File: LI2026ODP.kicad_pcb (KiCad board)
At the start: 4 copper layers, 19.8 x 40.1 mm, 33 parts, among them J1 9-1437539-2, J2 Conn_01x05_Male, U1 LM2936MPX-3.0_NOPB, U2 STM32G0B1KET6, U3 max6921aui

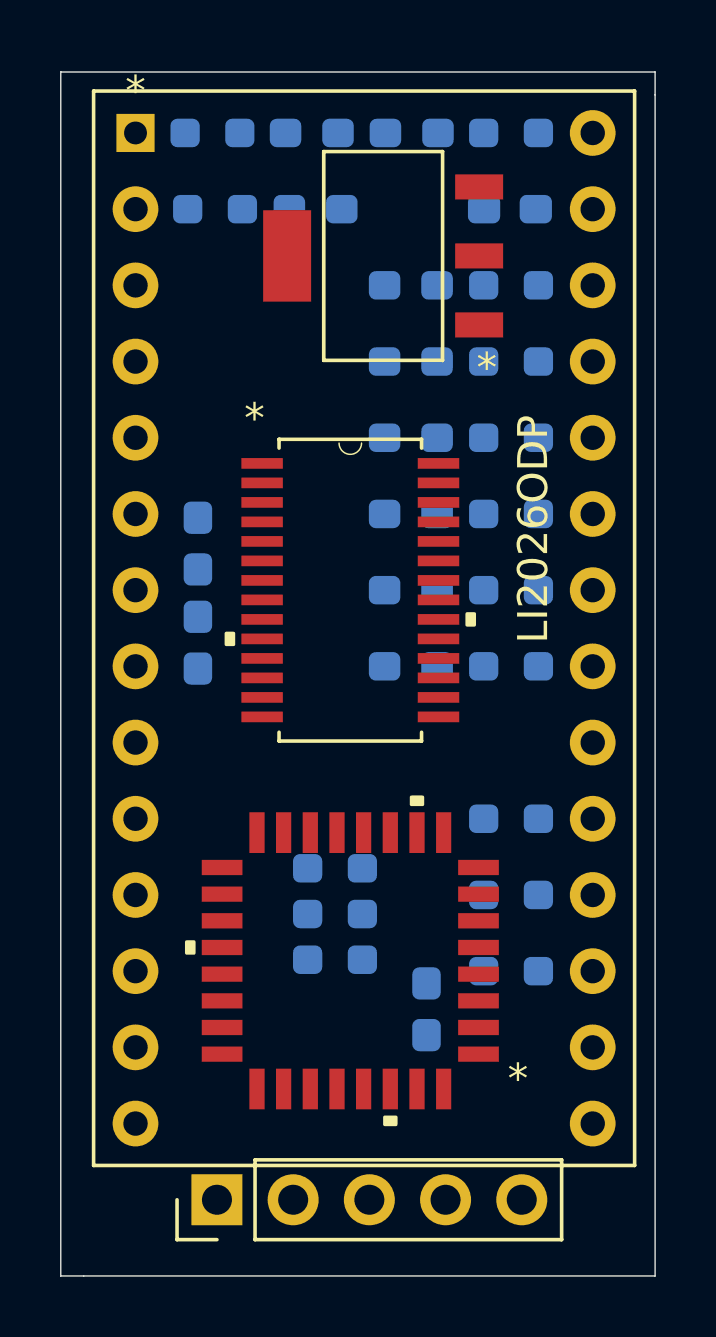
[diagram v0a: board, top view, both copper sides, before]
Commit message: layout finished.
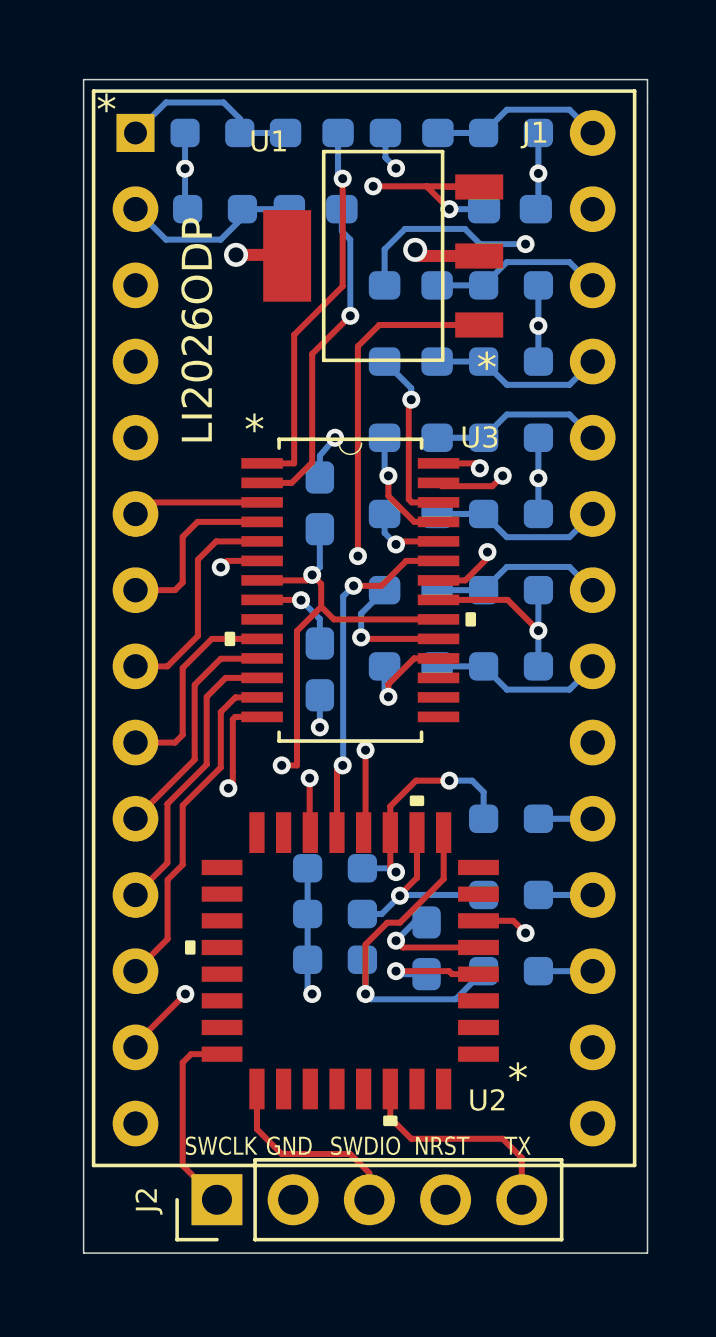
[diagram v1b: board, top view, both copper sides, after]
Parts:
- moved C3 4.28 mm to (123.4, 98.7)
- moved C2 4.16 mm to (123.4, 104.2)
- moved C4 2.03 mm to (127.0, 113.5), turned to 90 degrees
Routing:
- net +3V3: track 0.00 -> 47.8 mm, vias 0 -> 5
- net /+25V: track 0.00 -> 37.0 mm, vias 0 -> 2
- net GND: track 0.00 -> 31.5 mm, vias 0 -> 11
- net /D3: track 0.00 -> 16.8 mm, vias 0 -> 2
- net /D2: track 0.00 -> 13.9 mm, vias 0 -> 2
- net /SEG_DP: track 0.00 -> 13.3 mm, vias 0 -> 2
- net /SCK: track 0.00 -> 13.2 mm, vias 0 -> 2
- net /D1: track 0.00 -> 12.8 mm, vias 0 -> 1
- net /RKEY1: track 0.00 -> 12.3 mm, vias 0 -> 1
- net /NRST: track 0.00 -> 11.7 mm, vias 0 -> 1
- net /LOAD: track 0.00 -> 11.6 mm, vias 0 -> 2
- net /MOSI: track 0.00 -> 11.5 mm, vias 0 -> 2
- net /SEG_D: track 0.00 -> 11.4 mm
- net /D0: track 0.00 -> 11.0 mm, vias 0 -> 1
- net /SEG_C: track 0.00 -> 9.70 mm
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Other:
- board size 19.8 x 40.1 mm -> 18.8 x 39.1 mm
- net class Default: trace_width 0.25 -> 0.2; via_dia 0.8 -> 0.6; via_drill 0.4 -> 0.3
- rule via_min_size: 0.4 -> 0.5
- board text added: "GND"
- board text added: "NRST"
- board text added: "SWCLK"
- board text added: "SWDIO"
- board text added: "TX"
